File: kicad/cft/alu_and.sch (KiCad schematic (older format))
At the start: 14 parts, among them U1507 74HC541, U1508 74HC541, U2801 74HC08, U2802 74HC08, U2803 74HC08, U2804 74HC08, U2805 74HC541, U2806 74HC541

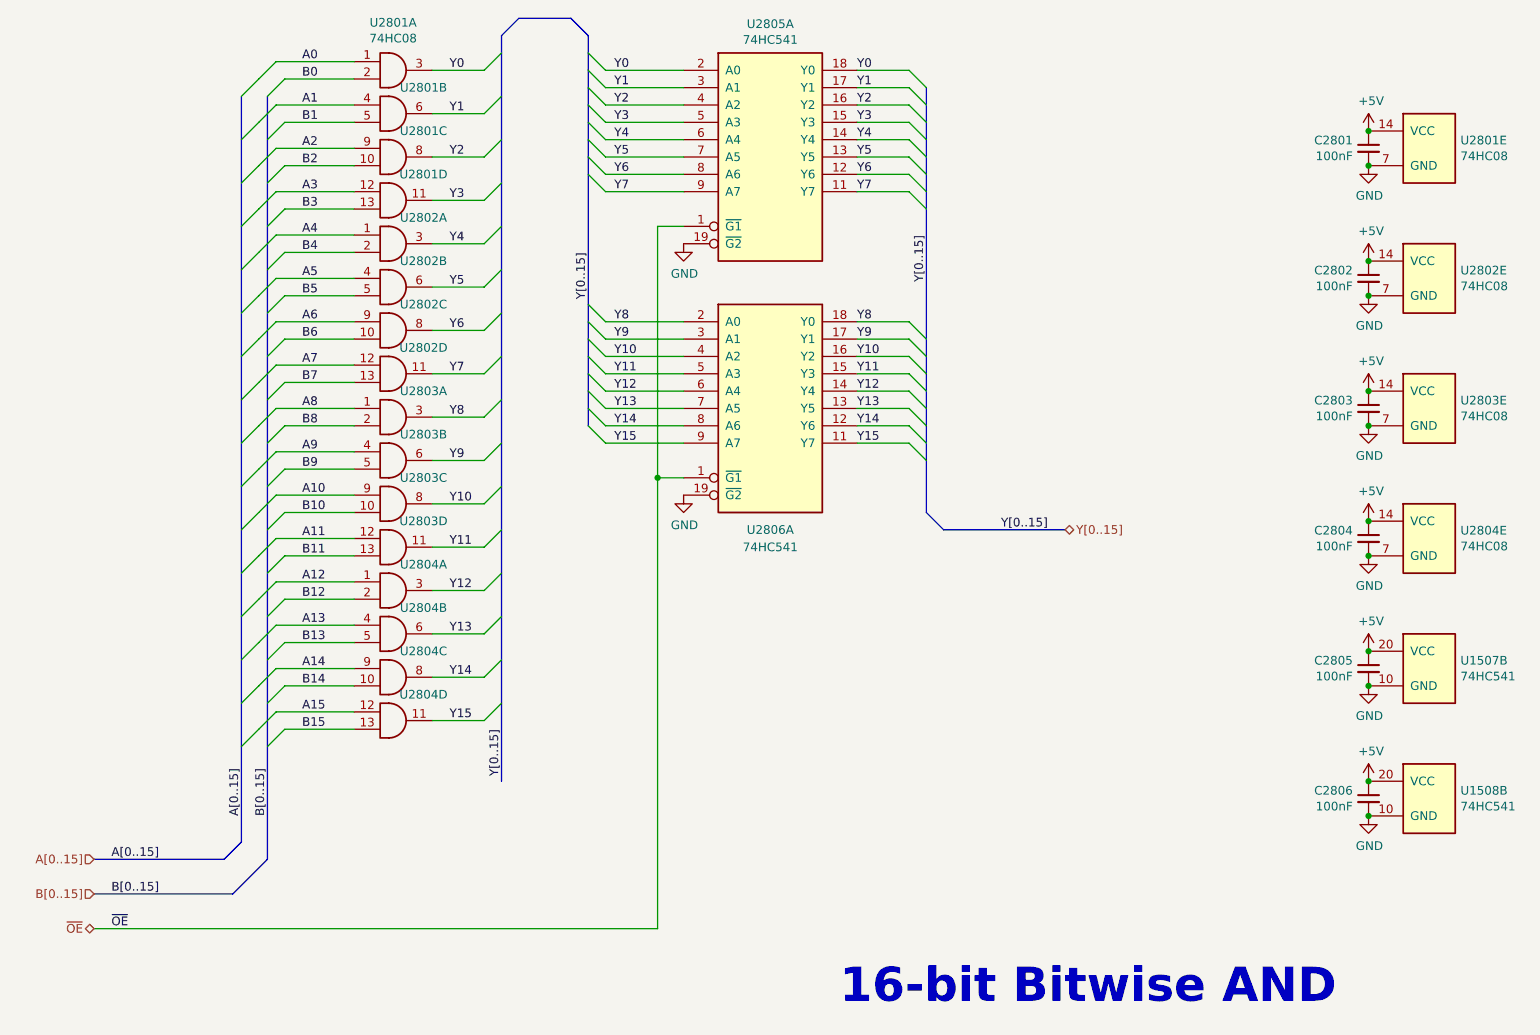
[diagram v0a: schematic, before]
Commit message: Moved things around a bit
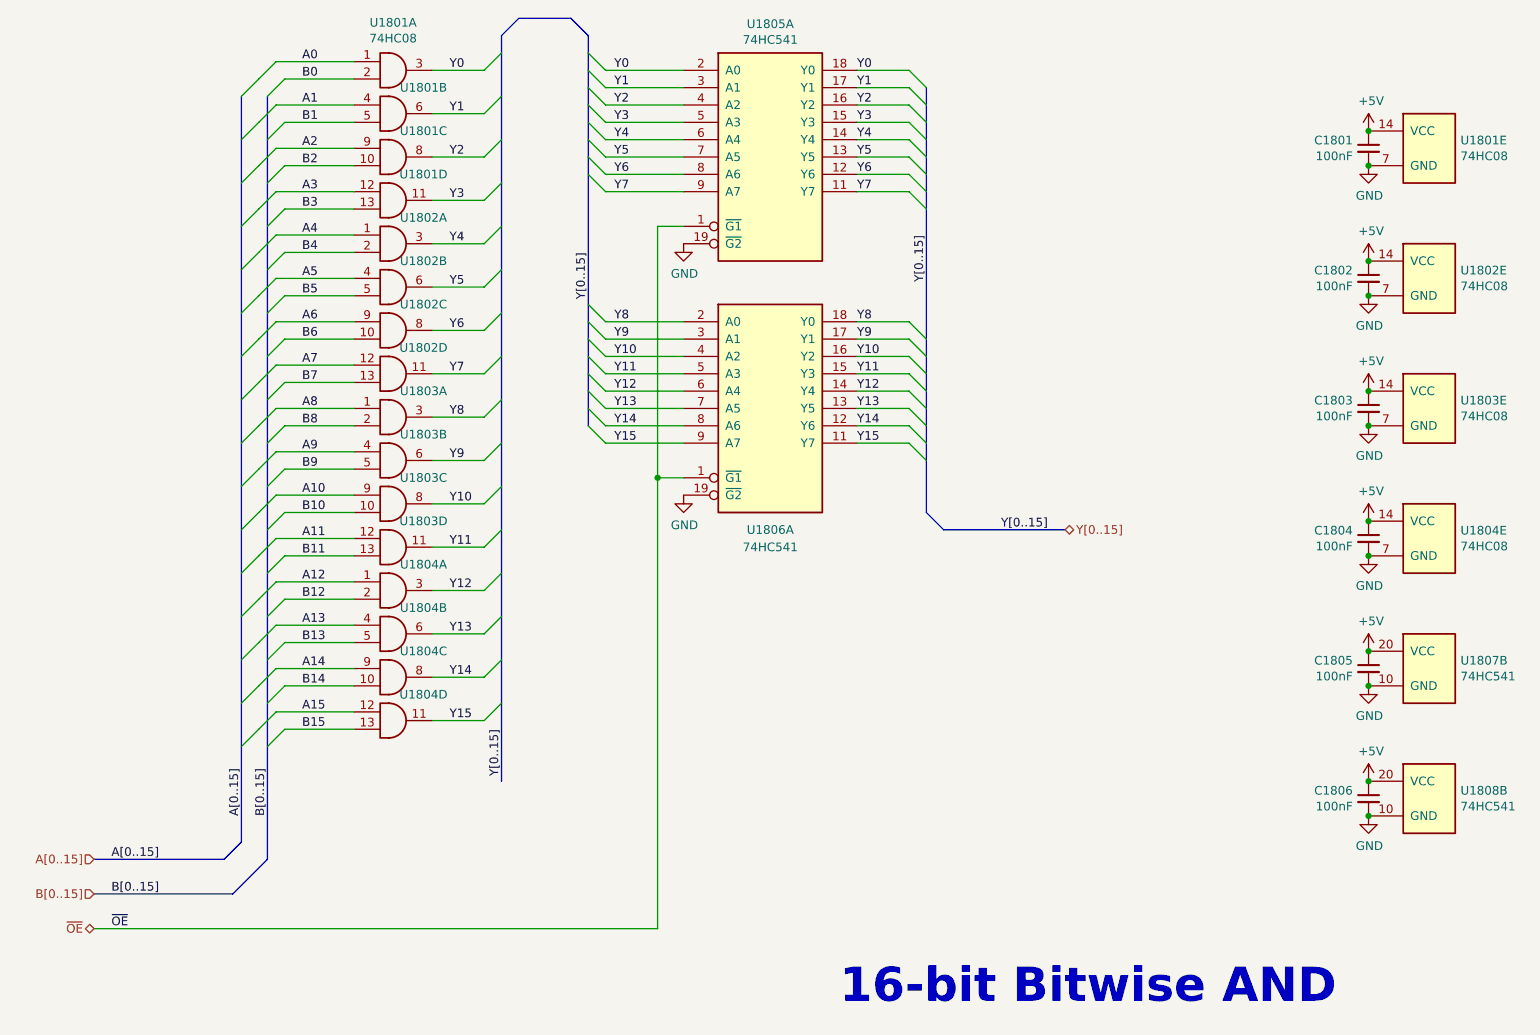
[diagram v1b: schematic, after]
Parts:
- renumbered C2801 to C1801, C2802 to C1802, C2803 to C1803, C2804 to C1804, C2805 to C1805, C2806 to C1806, U2801 to U1801, U2802 to U1802, U2803 to U1803, U2804 to U1804, U2805 to U1805, U2806 to U1806, U1507 to U1807, U1508 to U1808

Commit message: Removed widebus buffer from microcode store µAddr High
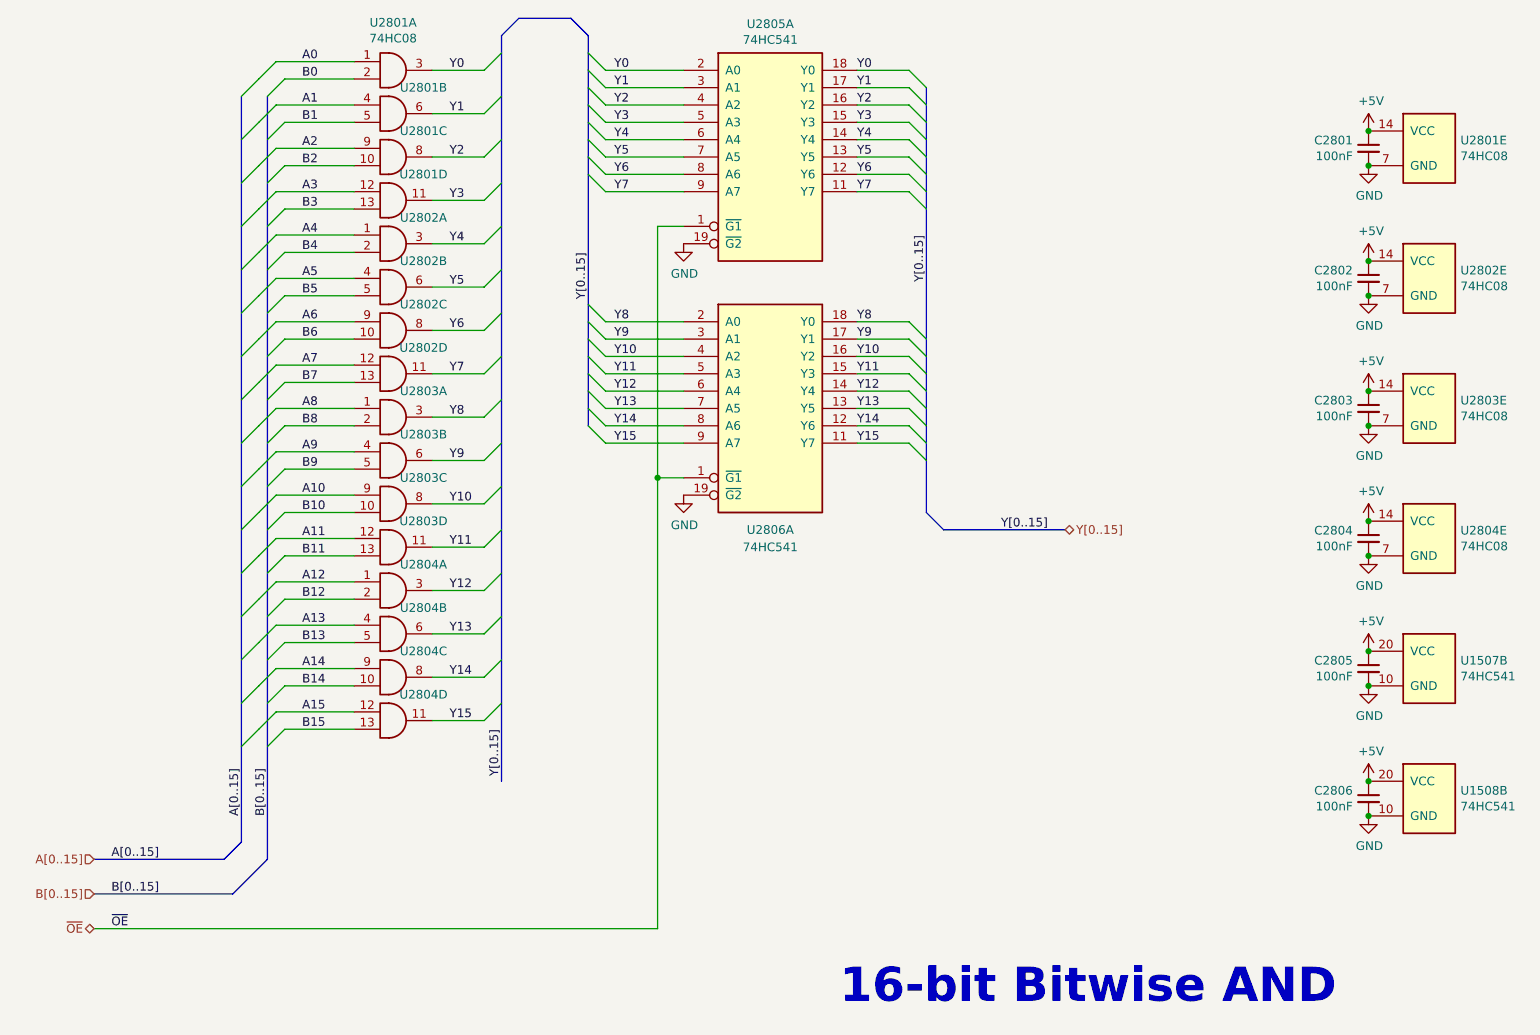
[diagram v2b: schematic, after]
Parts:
- renumbered C1801 to C2801, C1802 to C2802, C1803 to C2803, C1804 to C2804, C1805 to C2805, C1806 to C2806, U1807 to U1507, U1808 to U1508, U1801 to U2801, U1802 to U2802, U1803 to U2803, U1804 to U2804, U1805 to U2805, U1806 to U2806
